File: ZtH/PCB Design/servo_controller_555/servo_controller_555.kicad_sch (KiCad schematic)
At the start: 21 parts, among them J1 SERVO, J2 VIN, U1 LM555xN, U2 AMS1117

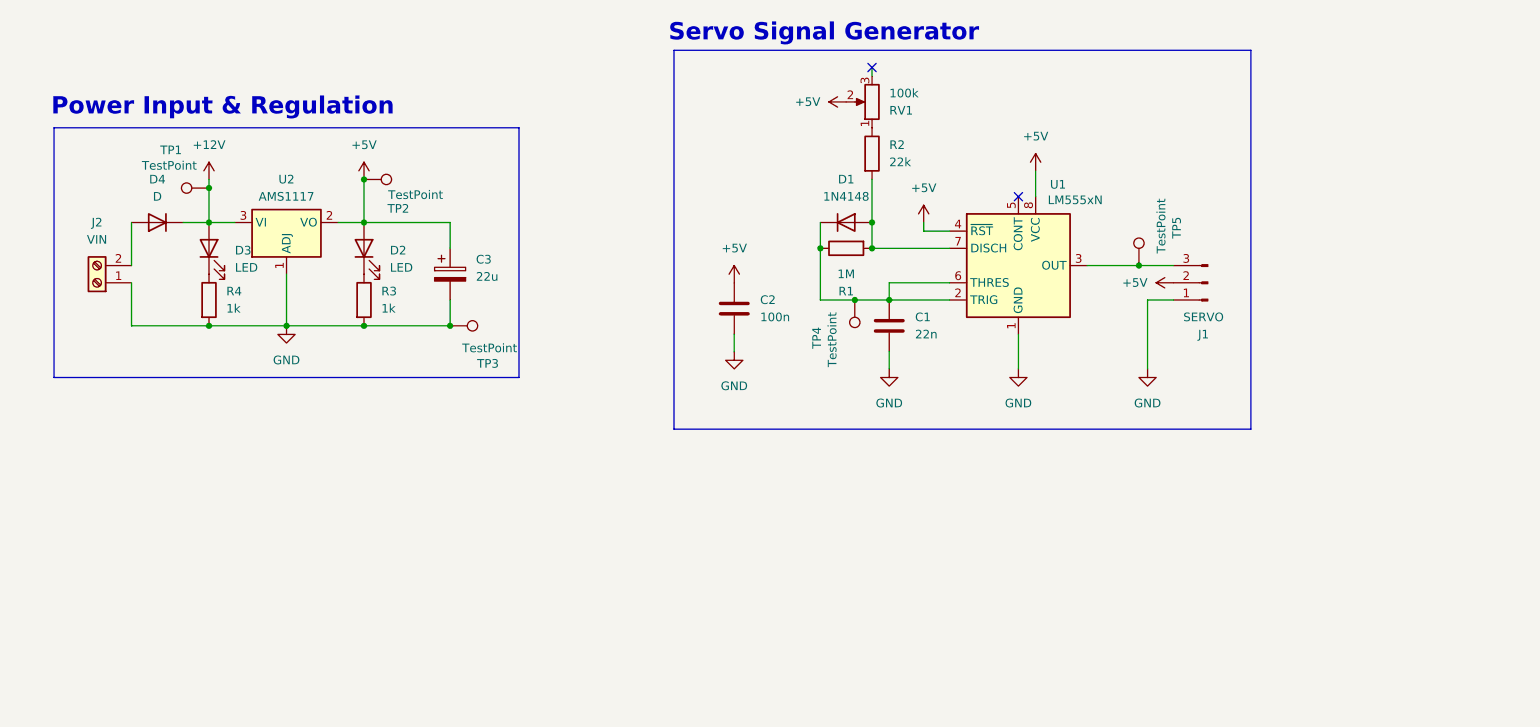
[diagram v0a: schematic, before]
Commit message: PCB and Lab Tools Complete
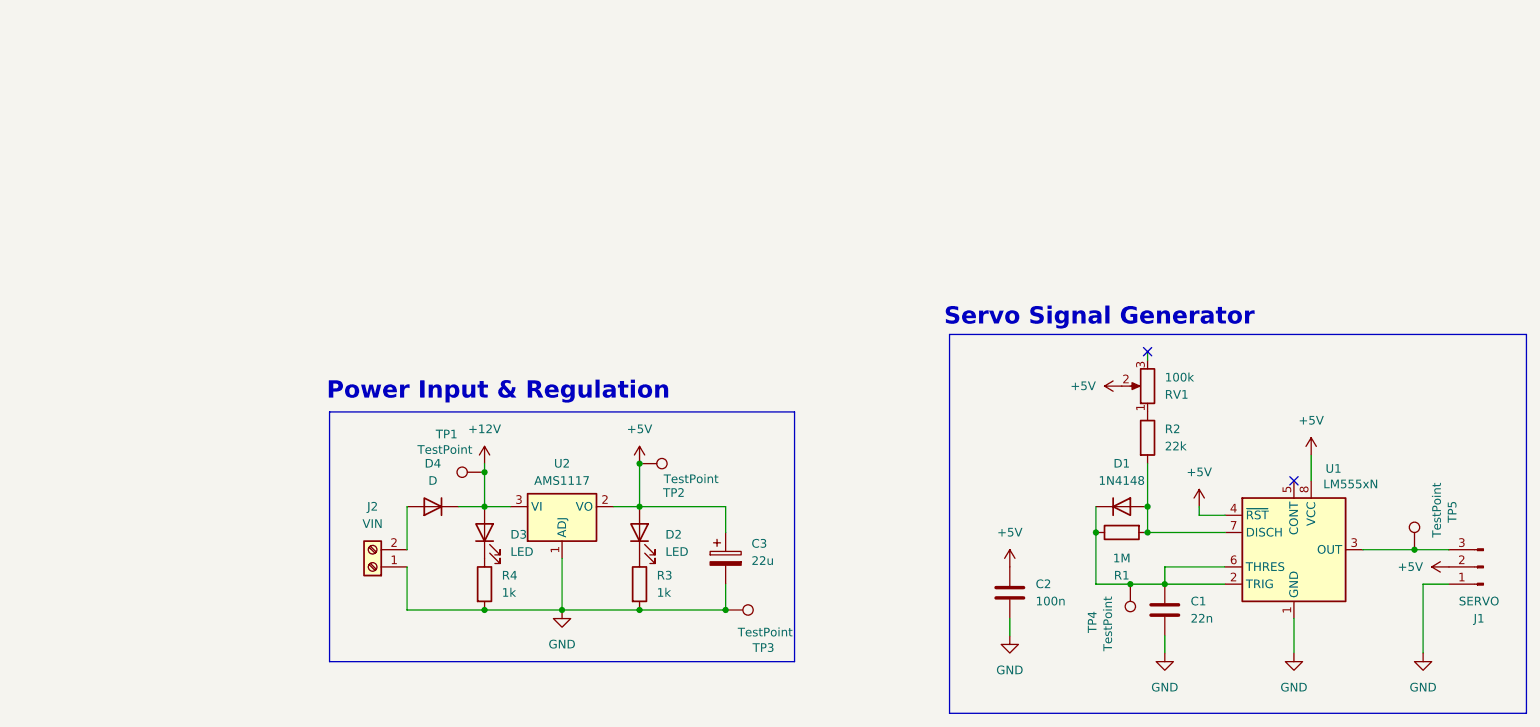
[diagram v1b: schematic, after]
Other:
- moved on the sheet: C1, C2, C3, D1, D2, D3, D4, J1, J2, R1, R2, R3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

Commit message: finish pcb frfr ong
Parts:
- TP1, TP2, TP4, TP5: footprint (none) -> TestPoint:TestPoint_THTPad_D2.0mm_Drill1.0mm
- TP3: footprint (none) -> TestPoint:TestPoint_Pad_4.0x4.0mm
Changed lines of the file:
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@@
 			)
 		)
-		(property "Footprint" ""
+		(property "Footprint" "TestPoint:TestPoint_Pad_4.0x4.0mm"
 			(at 160.02 149.86 0)
 			(hide yes)
@@
 			)
 		)
-		(property "Footprint" ""
+		(property "Footprint" "TestPoint:TestPoint_THTPad_D2.0mm_Drill1.0mm"
 			(at 147.32 128.27 0)
 			(hide yes)
@@
 			)
 		)
-		(property "Footprint" ""
+		(property "Footprint" "TestPoint:TestPoint_THTPad_D2.0mm_Drill1.0mm"
 			(at 266.7 135.89 0)
 			(hide yes)
@@
 			)
 		)
-		(property "Footprint" ""
+		(property "Footprint" "TestPoint:TestPoint_THTPad_D2.0mm_Drill1.0mm"
 			(at 214.63 140.97 0)
 			(hide yes)
@@
 			)
 		)
-		(property "Footprint" ""
+		(property "Footprint" "TestPoint:TestPoint_THTPad_D2.0mm_Drill1.0mm"
 			(at 124.46 119.38 0)
 			(hide yes)
